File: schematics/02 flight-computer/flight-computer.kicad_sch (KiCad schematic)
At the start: 46 parts, among them J1 SWD, J2 PWR, J3 GND CTRL, J4 RADIO, J5 PYRO, J6 DATALOGGER, J7 BLACKBOX, U1 MAX14787E, U2 STM32F405RGT6, U3 MAX14787E, Y1 26M

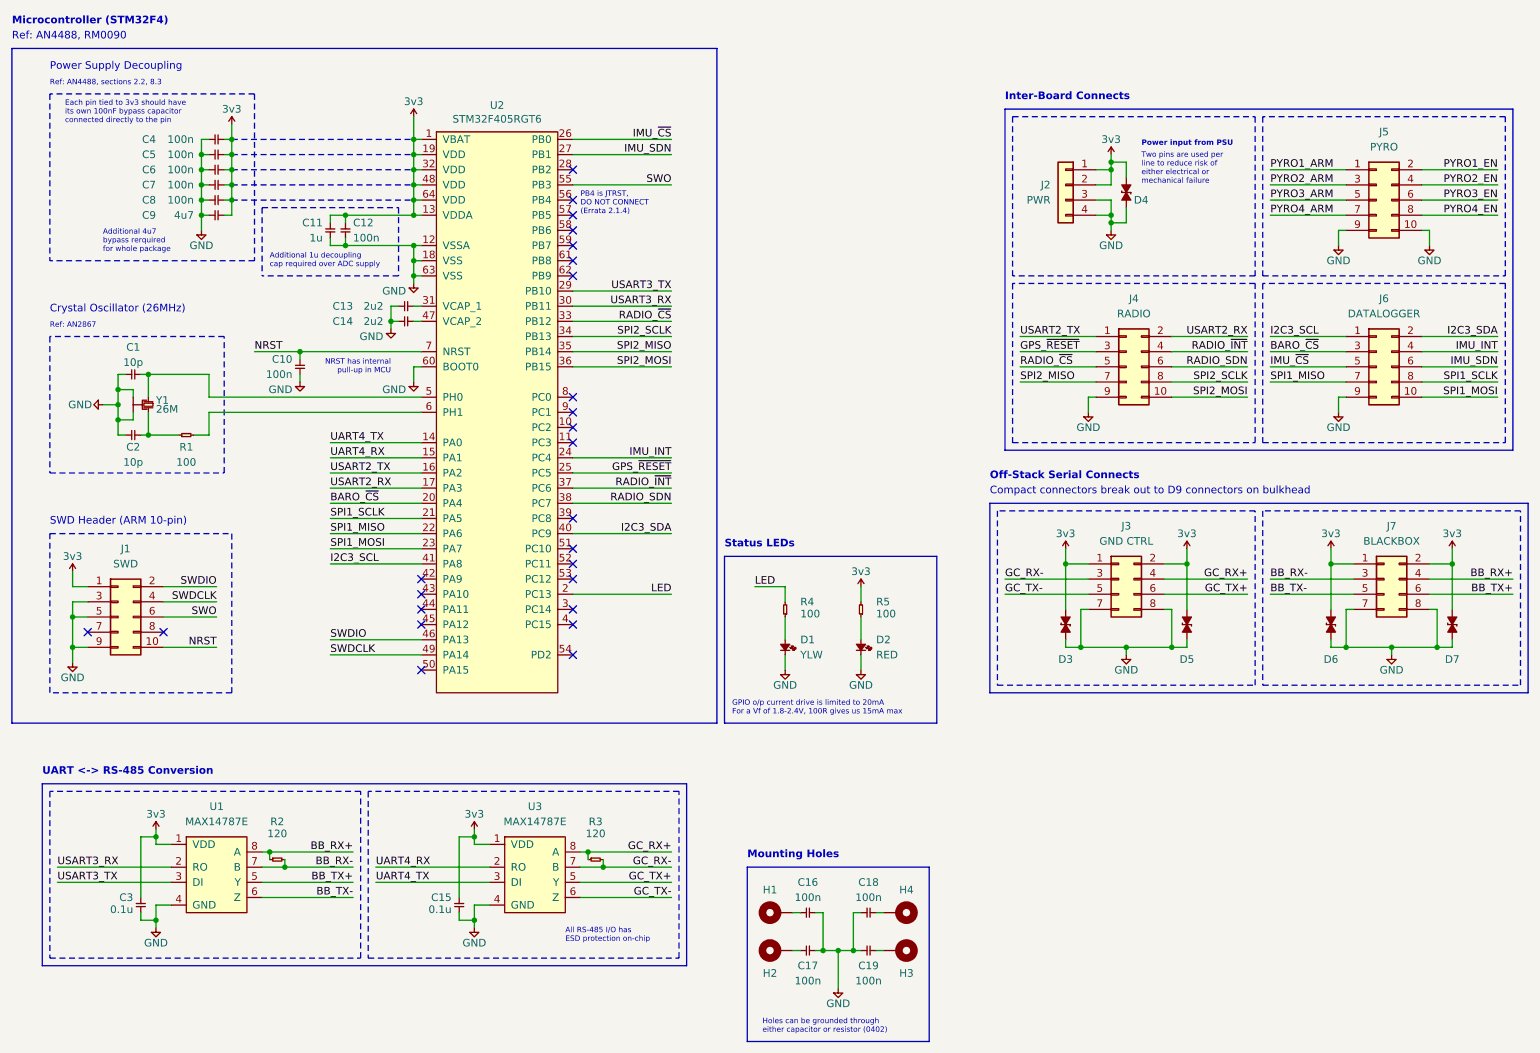
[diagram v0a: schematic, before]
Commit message: Further schematic work
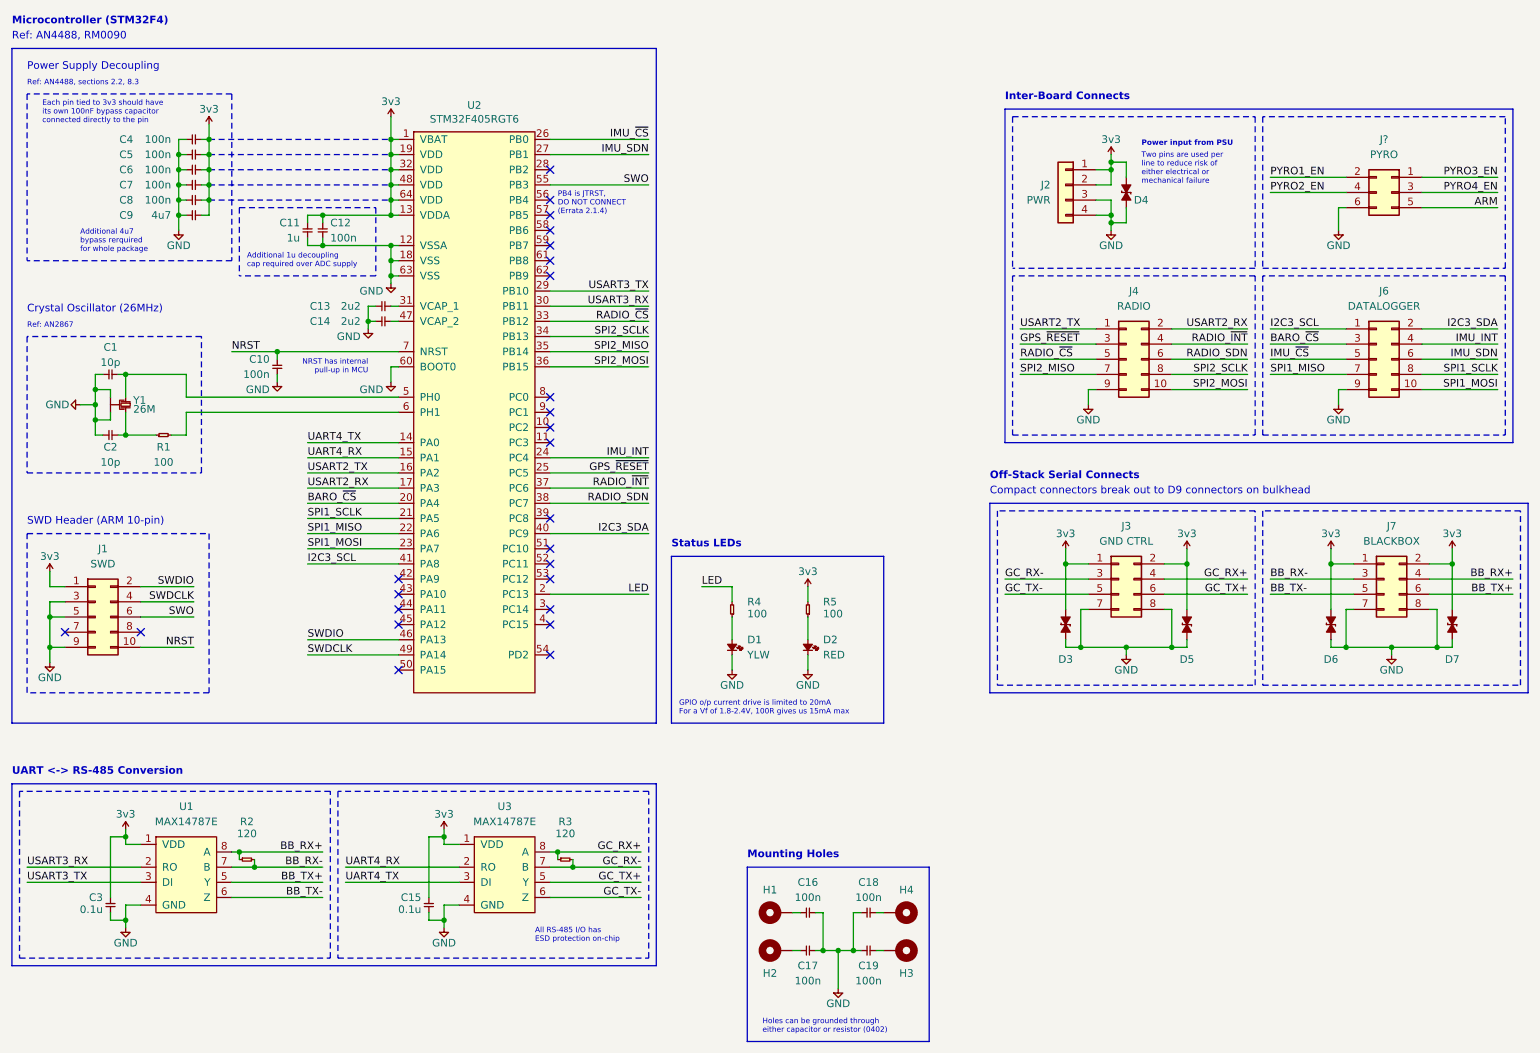
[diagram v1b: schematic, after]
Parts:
- removed J5: PYRO, Strix:Molex_Nano-Fit_105314-1110, symbol Strix:Conn_02x05
- added J?: PYRO, symbol Strix:Conn_02x03
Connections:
- net GND: now also J?.6 (Pin_6)
- net PYRO1_EN: now also J?.2 (Pin_2)
- net PYRO2_EN: now also J?.4 (Pin_4)
- net PYRO3_EN: now also J?.1 (Pin_1)
- net PYRO4_EN: now also J?.3 (Pin_3)
- new net ARM: J?.5 (Pin_5)
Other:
- moved on the sheet: C1, C10, C11, C12, C13, C14, C15, C2, C3, C4, C5, C6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
